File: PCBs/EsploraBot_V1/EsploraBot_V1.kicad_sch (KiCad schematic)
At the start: 16 parts, among them J1 HMC5883L, J2 VL53L0X_IZQ, J3 VL53L0X_DER, J4 HC-SR04, J5 Batería, J6 MotorIzq, J7 MotorDer, SW1 SW_SPDT, U1 ESP32-DEVKIT-V1, U2 TB6612FNG_1, U3 module_mpu6050, U4 LM2596

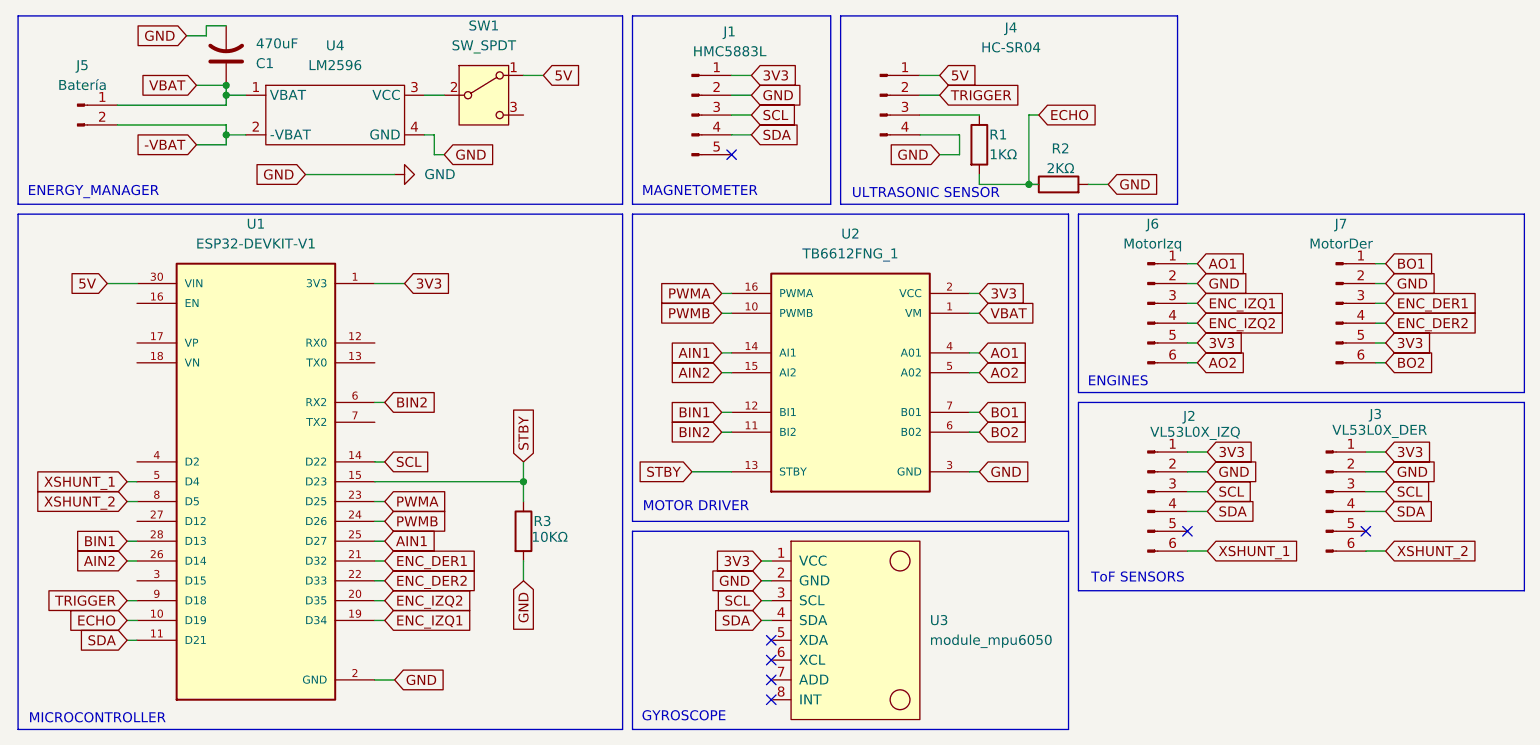
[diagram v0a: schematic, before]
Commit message: fix: Se realizaron algunos ajuste esteticos en el esquematico y PCB
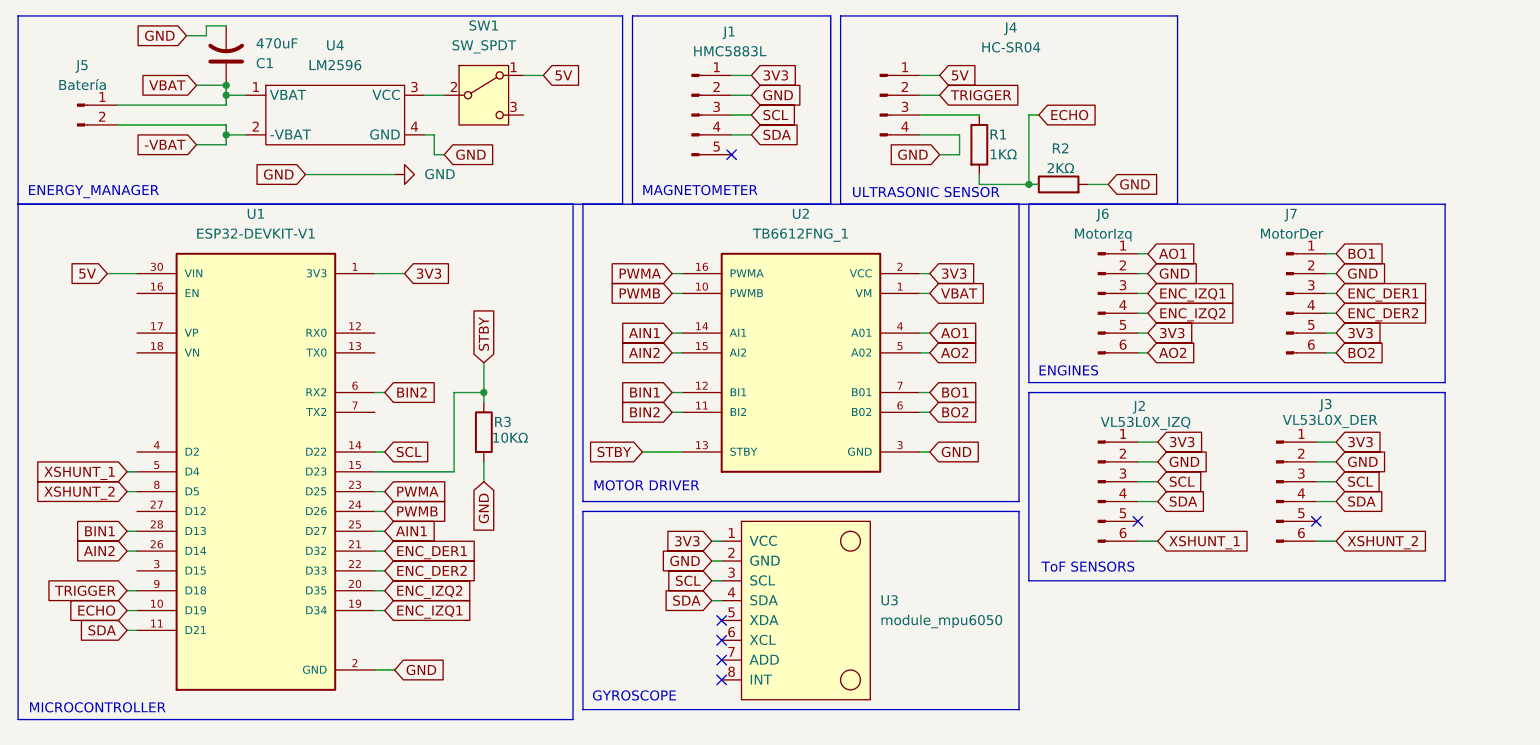
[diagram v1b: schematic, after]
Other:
- company: (none) -> Pavo's RoboticProjects
- title: (none) -> ExploraBot_V1
- moved on the sheet: J2, J3, J6, J7, R3, U1, U2, U3
